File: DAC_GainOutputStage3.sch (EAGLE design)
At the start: 69 parts, among them J1 1935190, J3 SJ-63033A, U1 V_REG_317SMD, U2 V_REG_317SMD

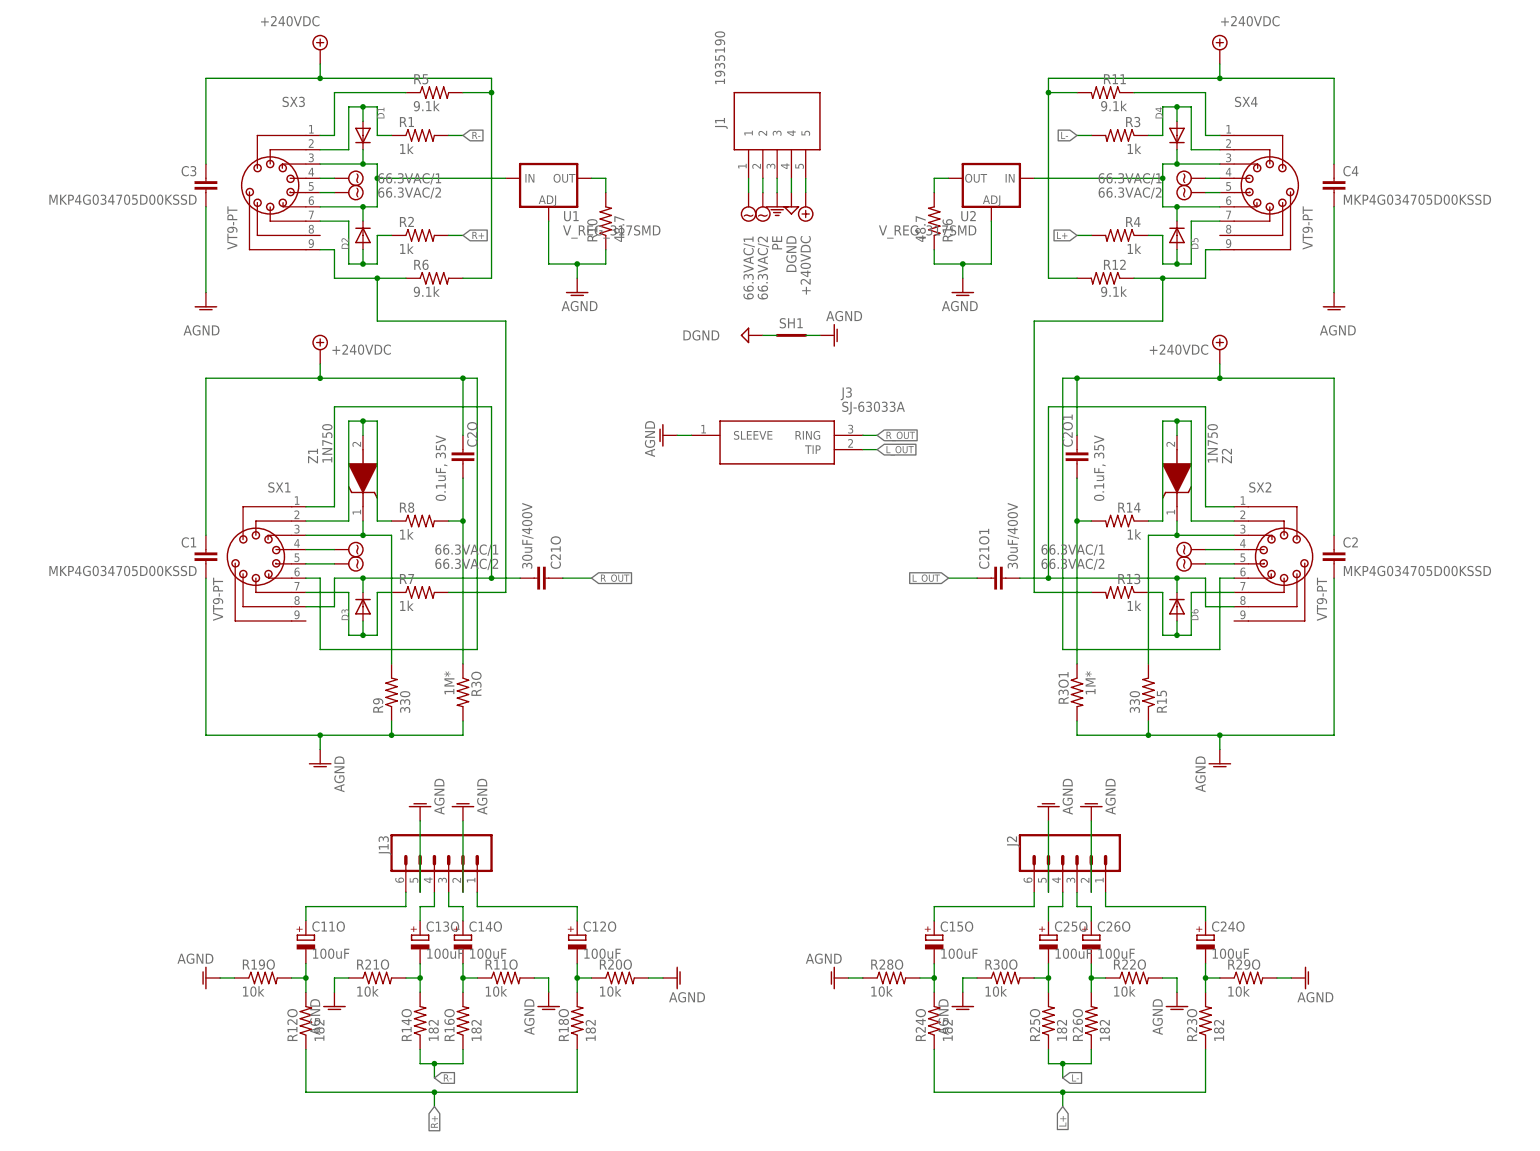
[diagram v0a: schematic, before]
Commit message: Finished routing
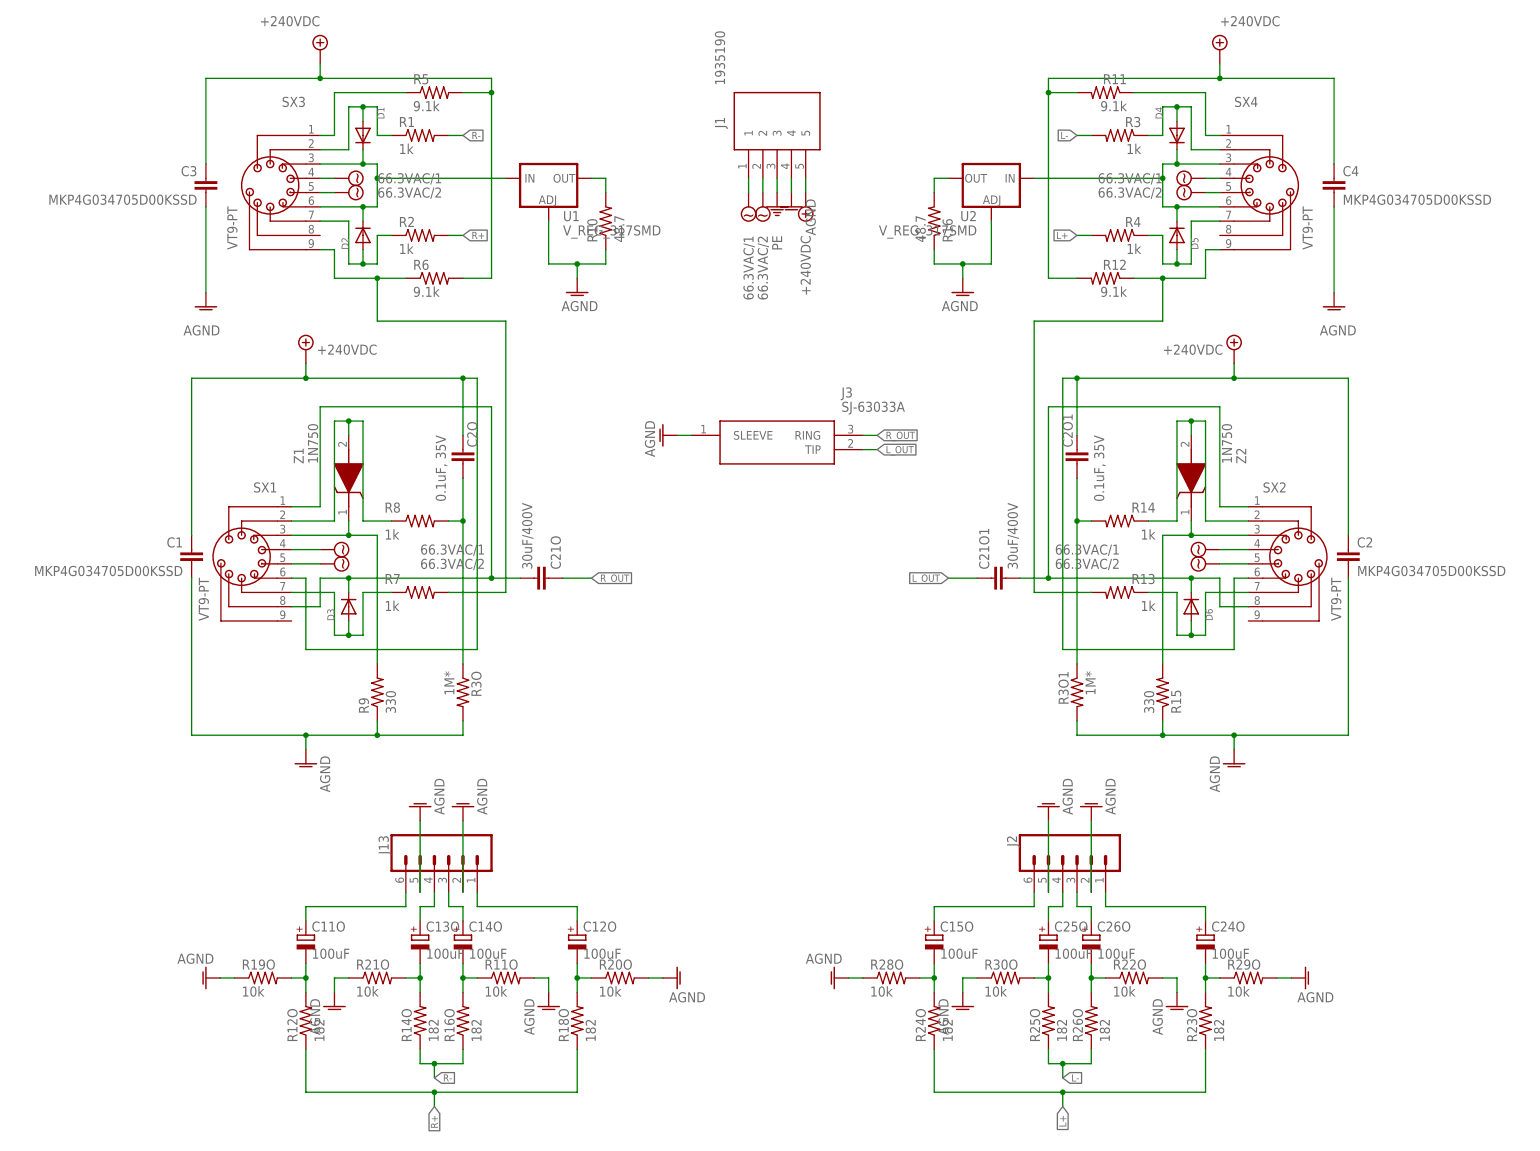
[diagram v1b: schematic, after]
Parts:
- removed SH1: SHORTA5, Dual Mono Amp Library:SHORTA5
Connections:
- removed net DGND: J1.4, SH1.P$1
- net AGND: now also J1.4; no longer SH1.P$2
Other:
- moved on the sheet: C1, C2, D3, D6, R15, R9, SX1, SX2, Z1, Z2

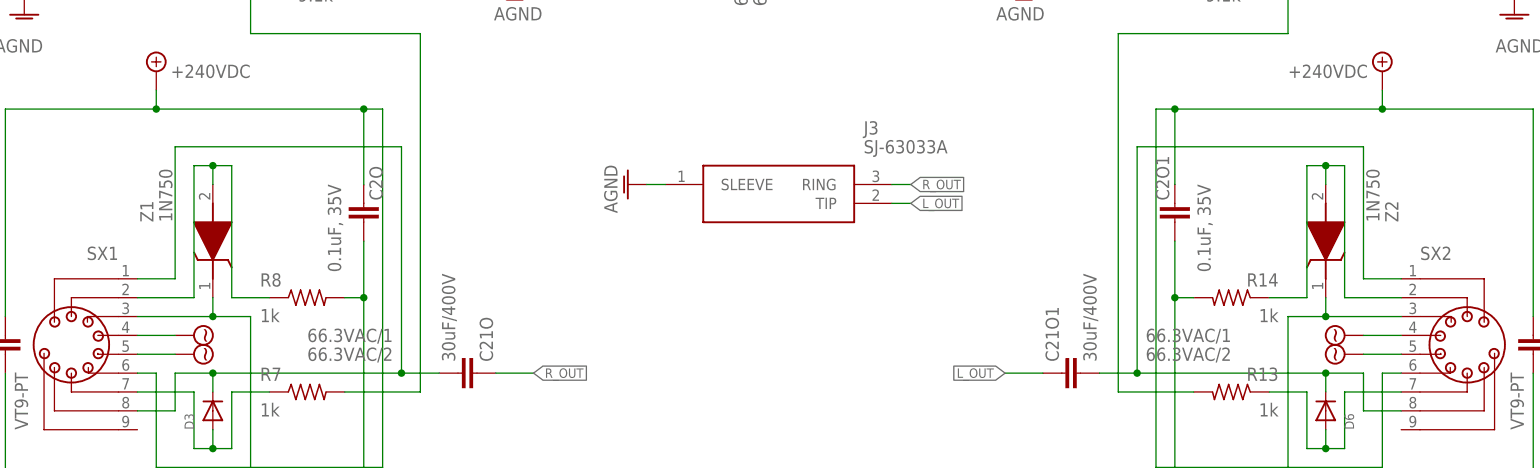
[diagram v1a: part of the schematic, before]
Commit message: Progress
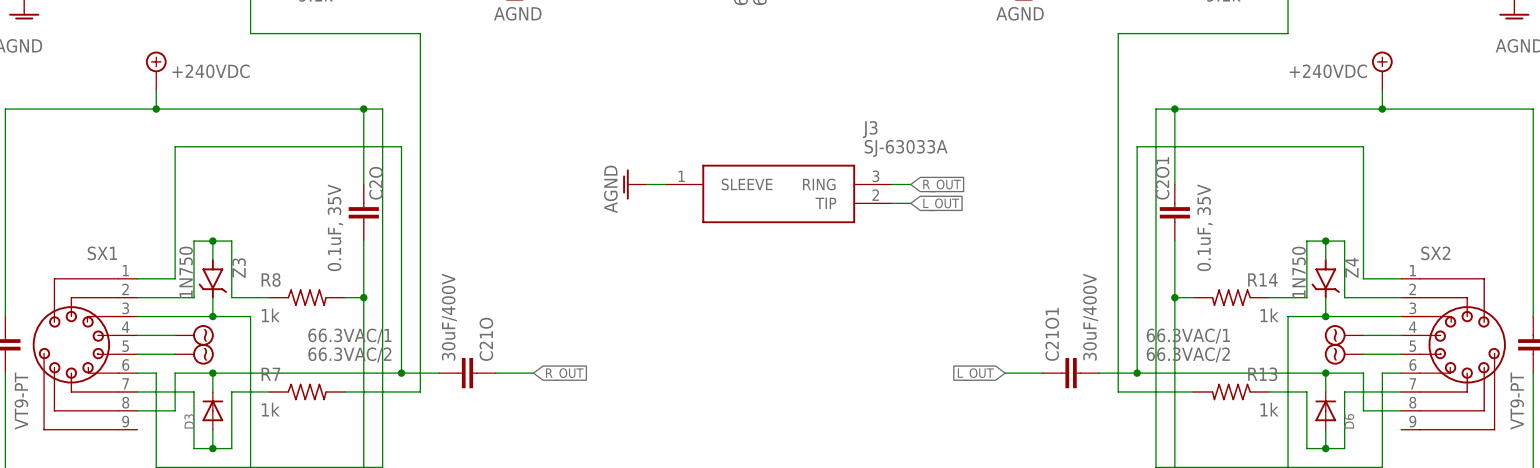
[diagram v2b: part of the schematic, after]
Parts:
- removed Z1, Z2: 1N750, 1N750:1N750
- added Z3, Z4: 1N750, Dual Mono Amp Library:1N750
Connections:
- net N$14: now also Z4.A; no longer Z2.A
- net N$2: now also Z3.A; no longer Z1.A
- net N$26: now also Z3.C; no longer Z1.K
- net N$27: now also Z4.C; no longer Z2.K
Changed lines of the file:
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@@
 <part name="D2" library="adafruit" library_urn="urn:adsk.eagle:library:420" deviceset="DIODE" device="DO-1N4148" package3d_urn="urn:adsk.eagle:package:6240748/1"/>
 <part name="D3" library="adafruit" library_urn="urn:adsk.eagle:library:420" deviceset="DIODE" device="DO-1N4148" package3d_urn="urn:adsk.eagle:package:6240748/1"/>
-<part name="Z1" library="1N750" deviceset="1N750" device=""/>
 <part name="U1" library="SparkFun-IC-Power" library_urn="urn:adsk.eagle:library:526" deviceset="V_REG_317" device="SMD" package3d_urn="urn:adsk.eagle:package:39069/2"/>
 <part name="R10" library="rcl" library_urn="urn:adsk.eagle:library:334" deviceset="R-US_" device="0207/10" package3d_urn="urn:adsk.eagle:package:23491/2" value="48.7"/>
@@
 <part name="D5" library="adafruit" library_urn="urn:adsk.eagle:library:420" deviceset="DIODE" device="DO-1N4148" package3d_urn="urn:adsk.eagle:package:6240748/1"/>
 <part name="D6" library="adafruit" library_urn="urn:adsk.eagle:library:420" deviceset="DIODE" device="DO-1N4148" package3d_urn="urn:adsk.eagle:package:6240748/1"/>
-<part name="Z2" library="1N750" deviceset="1N750" device=""/>
 <part name="U2" library="SparkFun-IC-Power" library_urn="urn:adsk.eagle:library:526" deviceset="V_REG_317" device="SMD" package3d_urn="urn:adsk.eagle:package:39069/2"/>
 <part name="R16" library="rcl" library_urn="urn:adsk.eagle:library:334" deviceset="R-US_" device="0207/10" package3d_urn="urn:adsk.eagle:package:23491/2" value="48.7"/>
 <part name="AGND19" library="Dual Mono Amp Library" library_urn="urn:adsk.wipprod:fs.file:vf.VjdQUjkvQKmMNRW9J90YWw" deviceset="AGND" device=""/>
+<part name="Z3" library="Dual Mono Amp Library" library_urn="urn:adsk.eagle:library:47621477" deviceset="1N750" device="" package3d_urn="urn:adsk.eagle:package:48500160/1"/>
+<part name="Z4" library="Dual Mono Amp Library" library_urn="urn:adsk.eagle:library:47621477" deviceset="1N750" device="" package3d_urn="urn:adsk.eagle:package:48500160/1"/>
 </parts>
 <sheets>
@@
 <attribute name="VALUE" x="29.21" y="114.3" size="1.27" layer="96" rot="R90"/>
 </instance>
-<instance part="Z1" gate="G$1" x="25.4" y="132.08" smashed="yes" rot="R90">
-<attribute name="NAME" x="16.51" y="142.24" size="1.778" layer="95" rot="R90" align="center-left"/>
-<attribute name="VALUE" x="19.05" y="142.24" size="1.778" layer="96" rot="R90" align="center-left"/>
-</instance>
 <instance part="U1" gate="G$1" x="60.96" y="193.04" smashed="yes">
 <attribute name="NAME" x="63.5" y="185.42" size="1.778" layer="95"/>
@@
 <attribute name="VALUE" x="171.45" y="114.3" size="1.27" layer="96" rot="MR90"/>
 </instance>
-<instance part="Z2" gate="G$1" x="175.26" y="132.08" smashed="yes" rot="MR90">
-<attribute name="NAME" x="184.15" y="142.24" size="1.778" layer="95" rot="MR90" align="center-left"/>
-<attribute name="VALUE" x="181.61" y="142.24" size="1.778" layer="96" rot="MR90" align="center-left"/>
-</instance>
 <instance part="U2" gate="G$1" x="139.7" y="193.04" smashed="yes" rot="MR0">
 <attribute name="NAME" x="137.16" y="185.42" size="1.778" layer="95" rot="MR0"/>
@@
 <instance part="AGND19" gate="VR1" x="134.62" y="172.72" smashed="yes">
 <attribute name="VALUE" x="137.414" y="169.418" size="1.778" layer="96" rot="MR0"/>
+</instance>
+<instance part="Z3" gate="G$1" x="25.4" y="134.62" smashed="yes" rot="R270">
+<attribute name="NAME" x="28.0416" y="137.5664" size="1.778" layer="95" rot="R270"/>
+<attribute name="VALUE" x="20.9042" y="139.0904" size="1.778" layer="96" rot="R270"/>
+</instance>
+<instance part="Z4" gate="G$1" x="175.26" y="134.62" smashed="yes" rot="R270">
+<attribute name="NAME" x="177.9016" y="137.5664" size="1.778" layer="95" rot="R270"/>
+<attribute name="VALUE" x="170.7642" y="139.0904" size="1.778" layer="96" rot="R270"/>
 </instance>
 </instances>
@@
 <pinref part="R8" gate="G$1" pin="1"/>
 <wire x1="33.02" y1="132.08" x2="27.94" y2="132.08" width="0.1524" layer="91"/>
-<wire x1="27.94" y1="132.08" x2="27.94" y2="149.86" width="0.1524" layer="91"/>
-<wire x1="27.94" y1="149.86" x2="25.4" y2="149.86" width="0.1524" layer="91"/>
-<wire x1="25.4" y1="149.86" x2="22.86" y2="149.86" width="0.1524" layer="91"/>
-<wire x1="22.86" y1="149.86" x2="22.86" y2="132.08" width="0.1524" layer="91"/>
+<wire x1="27.94" y1="132.08" x2="27.94" y2="139.7" width="0.1524" layer="91"/>
+<wire x1="27.94" y1="139.7" x2="25.4" y2="139.7" width="0.1524" layer="91"/>
+<wire x1="25.4" y1="139.7" x2="22.86" y2="139.7" width="0.1524" layer="91"/>
+<wire x1="22.86" y1="139.7" x2="22.86" y2="132.08" width="0.1524" layer="91"/>
 <wire x1="22.86" y1="132.08" x2="15.24" y2="132.08" width="0.1524" layer="91"/>
-<pinref part="Z1" gate="G$1" pin="A"/>
-<wire x1="25.4" y1="147.32" x2="25.4" y2="149.86" width="0.1524" layer="91"/>
-<junction x="25.4" y="149.86"/>
+<wire x1="25.4" y1="137.16" x2="25.4" y2="139.7" width="0.1524" layer="91"/>
+<junction x="25.4" y="139.7"/>
+<pinref part="Z3" gate="G$1" pin="A"/>
 </segment>
 </net>
@@
 <wire x1="25.4" y1="129.54" x2="30.48" y2="129.54" width="0.1524" layer="91"/>
 <wire x1="30.48" y1="129.54" x2="30.48" y2="106.68" width="0.1524" layer="91"/>
-<pinref part="Z1" gate="G$1" pin="K"/>
 <wire x1="25.4" y1="132.08" x2="25.4" y2="129.54" width="0.1524" layer="91"/>
 <junction x="25.4" y="129.54"/>
+<pinref part="Z3" gate="G$1" pin="C"/>
 </segment>
 </net>
@@
 <pinref part="R14" gate="G$1" pin="1"/>
 <wire x1="167.64" y1="132.08" x2="172.72" y2="132.08" width="0.1524" layer="91"/>
-<wire x1="172.72" y1="132.08" x2="172.72" y2="149.86" width="0.1524" layer="91"/>
-<wire x1="172.72" y1="149.86" x2="175.26" y2="149.86" width="0.1524" layer="91"/>
-<wire x1="175.26" y1="149.86" x2="177.8" y2="149.86" width="0.1524" layer="91"/>
-<wire x1="177.8" y1="149.86" x2="177.8" y2="132.08" width="0.1524" layer="91"/>
+<wire x1="172.72" y1="132.08" x2="172.72" y2="139.7" width="0.1524" layer="91"/>
+<wire x1="172.72" y1="139.7" x2="175.26" y2="139.7" width="0.1524" layer="91"/>
+<wire x1="175.26" y1="139.7" x2="177.8" y2="139.7" width="0.1524" layer="91"/>
+<wire x1="177.8" y1="139.7" x2="177.8" y2="132.08" width="0.1524" layer="91"/>
 <wire x1="177.8" y1="132.08" x2="185.42" y2="132.08" width="0.1524" layer="91"/>
-<pinref part="Z2" gate="G$1" pin="A"/>
-<wire x1="175.26" y1="147.32" x2="175.26" y2="149.86" width="0.1524" layer="91"/>
-<junction x="175.26" y="149.86"/>
+<wire x1="175.26" y1="137.16" x2="175.26" y2="139.7" width="0.1524" layer="91"/>
+<junction x="175.26" y="139.7"/>
+<pinref part="Z4" gate="G$1" pin="A"/>
 </segment>
 </net>
@@
 <wire x1="175.26" y1="129.54" x2="170.18" y2="129.54" width="0.1524" layer="91"/>
 <wire x1="170.18" y1="129.54" x2="170.18" y2="106.68" width="0.1524" layer="91"/>
-<pinref part="Z2" gate="G$1" pin="K"/>
 <wire x1="175.26" y1="132.08" x2="175.26" y2="129.54" width="0.1524" layer="91"/>
 <junction x="175.26" y="129.54"/>
-</segment>
-</net>
+<pinref part="Z4" gate="G$1" pin="C"/>
+</segment>
+</net>
